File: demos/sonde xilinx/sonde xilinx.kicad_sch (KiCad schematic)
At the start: 25 parts, among them J1 DB25MALE, J2 DB9MALE, P1 CONN_6, U1 74LS125, U2 74LS125

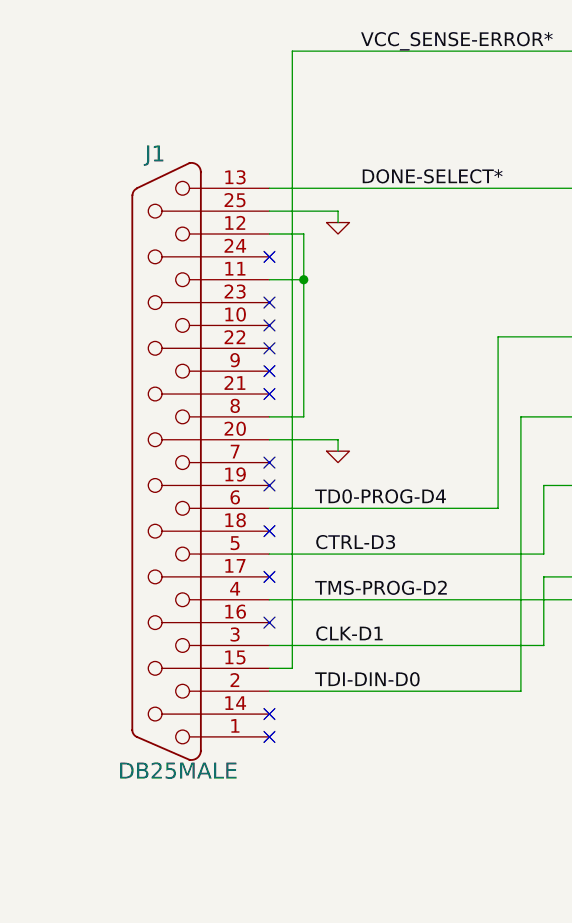
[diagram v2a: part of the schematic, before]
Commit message: Demos update
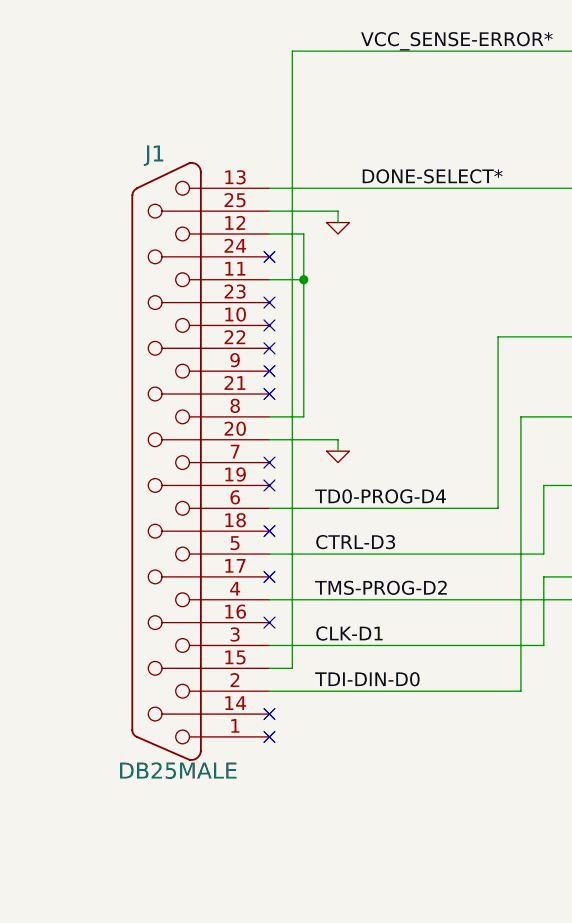
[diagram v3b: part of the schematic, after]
